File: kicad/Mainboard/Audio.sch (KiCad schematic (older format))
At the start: 45 parts, among them J10 SPK_INT, J11 SPK_EXT, J8 MIC_INT, J9 MIC_EXT, SW1 INT_PTT_SW, U7 OPA340UA, U8 LM386

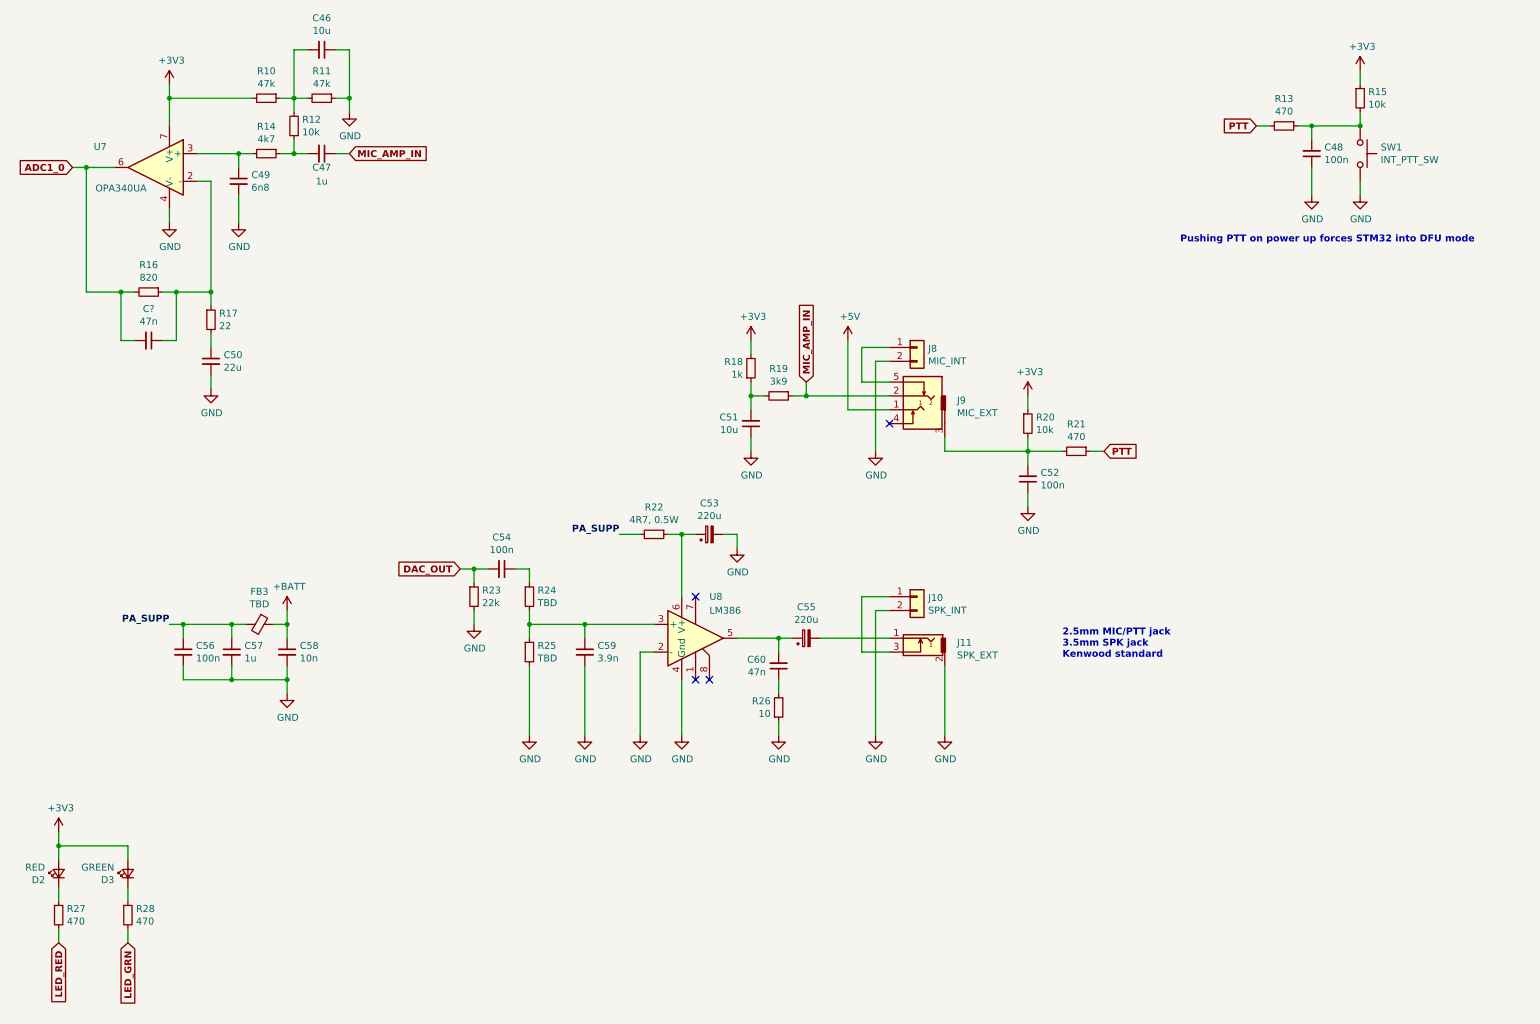
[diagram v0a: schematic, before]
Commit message: Add files via upload
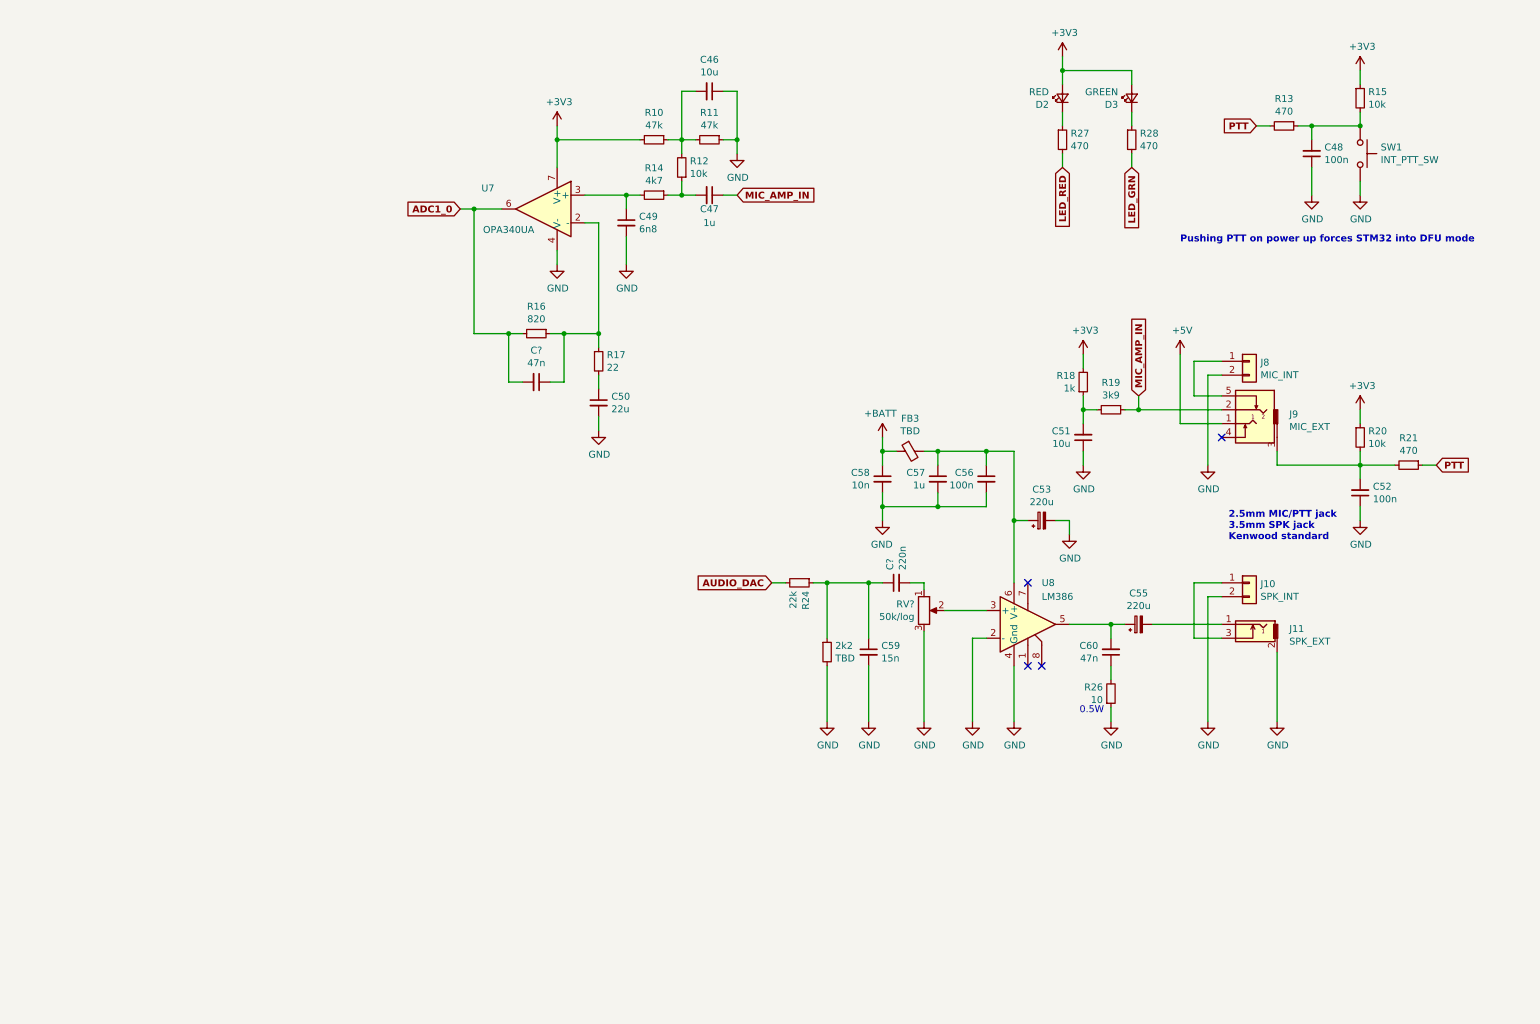
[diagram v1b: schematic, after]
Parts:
- removed C54: 100n, symbol Mainboard-rescue:C_Small-device
- removed R22: 4R7, 0.5W, symbol Mainboard-rescue:R_Small-device
- removed R23: 22k, symbol Mainboard-rescue:R_Small-device
- added C?: 220n, symbol Mainboard-rescue:C_Small-device
- added RV?: 50k/log, symbol Device:R_POT
- C59: value 3.9n -> 15n
- R24: value TBD -> 22k
- renumbered R25 to 2k2
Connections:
- net PA_SUPP is gone; now on an unnamed net: C56.1, C57.1, FB3.2
- net GND: now also RV?.3
- net at R24.1: now also 2k2.1, C59.1, C?.1
- new net: RV?.2, U8.3 (+)
- new net: C?.2, RV?.1
- new net AUDIO_DAC: R24.2
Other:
- note added: "0.5W"
- moved on the sheet: 2k2, C46, C47, C49, C50, C51, C52, C53, C55, C56, C57, C58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
